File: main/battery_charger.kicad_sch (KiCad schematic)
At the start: 52 parts, among them Q401 IXTP28P065T, Q402 TK4R3E06PL, Q403 IRLML0030, Q404 FDS6681Z, Q405 FDS6681Z, Q406 IRLML0030, U401 LT8710, U402 TMCS1101, U403 TSV911xxLx

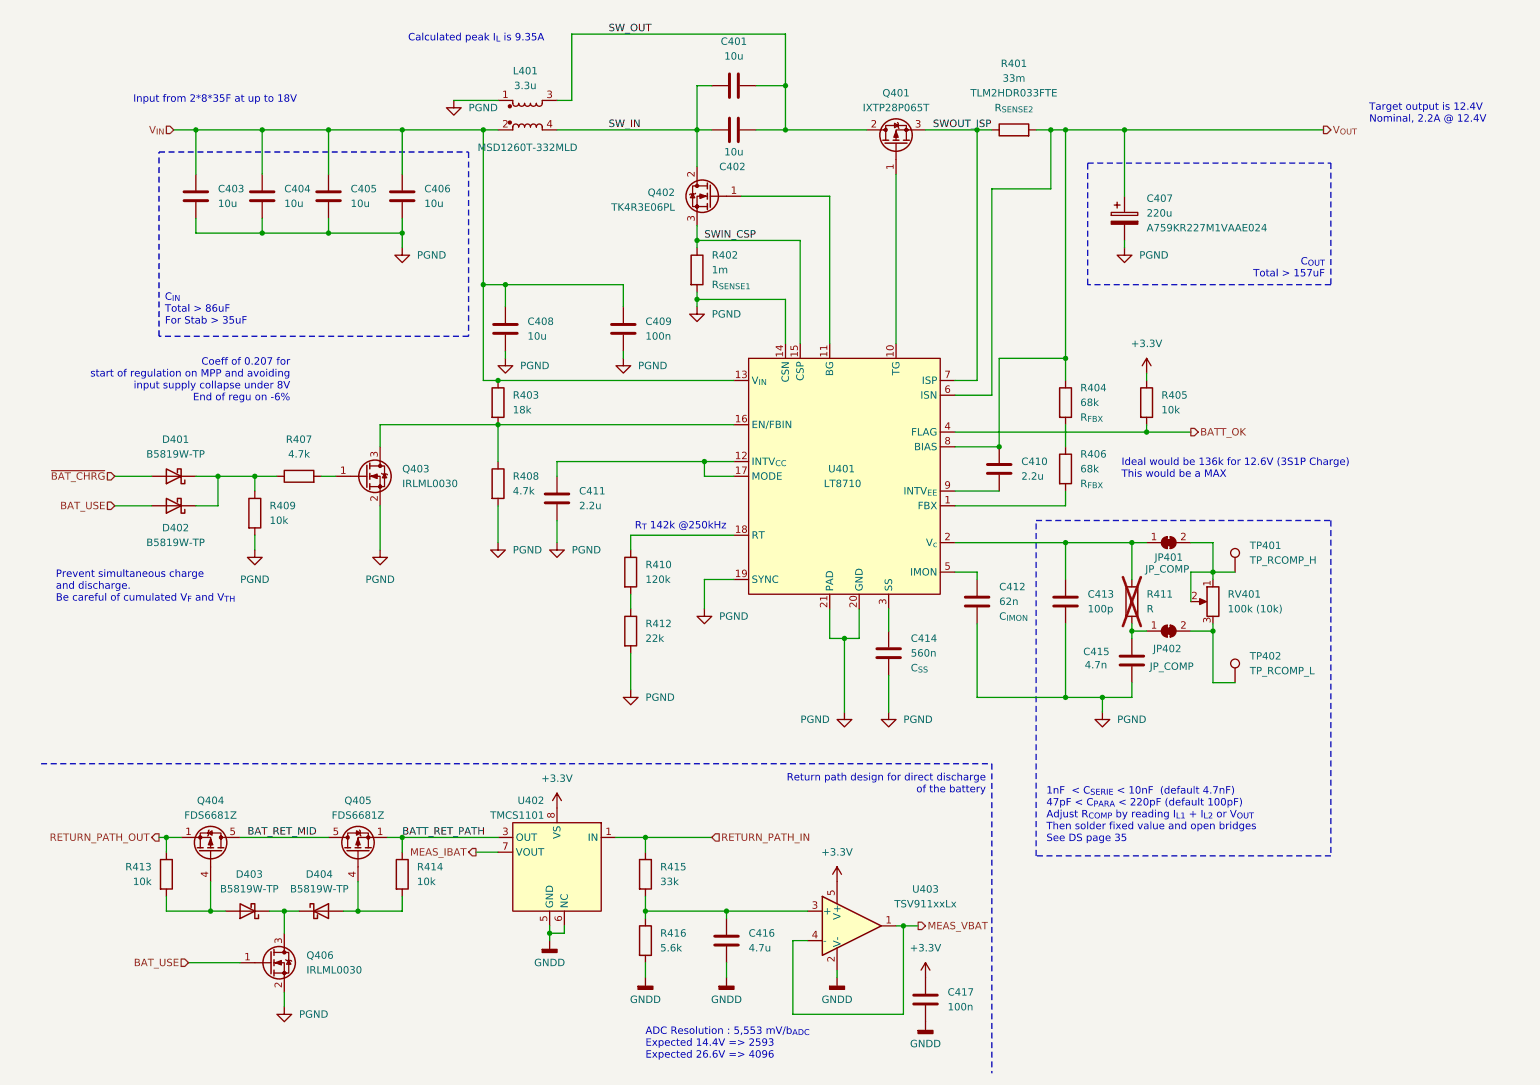
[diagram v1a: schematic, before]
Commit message: Sent to fab
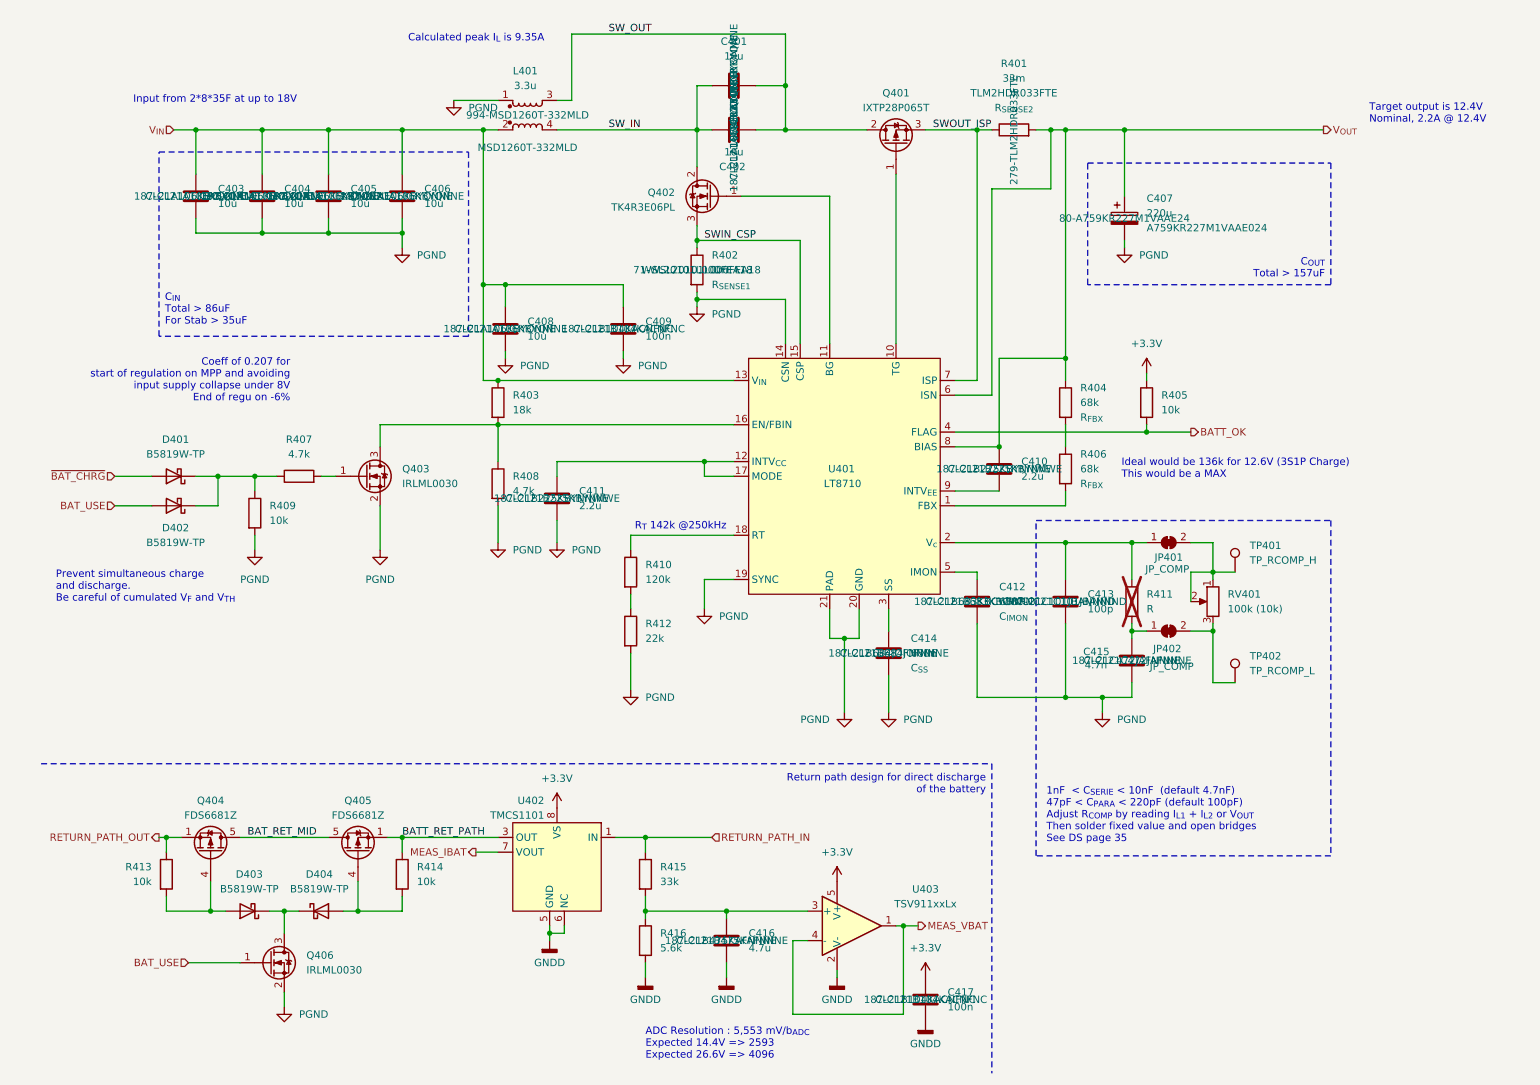
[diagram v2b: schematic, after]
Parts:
- C401, C402, C403, C404, C405, C406, C408: MPN (none) -> CL21A106KBYQNNE; Mouser SKU (none) -> 187-CL21A106KBYQNNE
- C407: Mouser SKU (none) -> 80-A759KR227M1VAAE24
- C409, C417: MPN (none) -> CL21B104KACNFNC; Mouser SKU (none) -> 187-CL21B104KACNFNC
- C410, C411: MPN (none) -> CL21B225KBYNNWE; Mouser SKU (none) -> 187-CL21B225KBYNNWE
- C412: value 62n -> 68n; MPN (none) -> CL21B683KBCWPNC; Mouser SKU (none) -> 187-CL21B683KBCWPNC
- C413: MPN (none) -> CL21C101JBANNND; Mouser SKU (none) -> 187-CL21C101JBANNND
- C414: value 560n -> 680n; MPN (none) -> CL21B684JOFNNNE; Mouser SKU (none) -> 187-CL21B684JOFNNNE
- C415: MPN (none) -> CL21C472JAFNNNE; Mouser SKU (none) -> 187-CL21C472JAFNNNE
- C416: MPN (none) -> CL21B475KAFNNNE; Mouser SKU (none) -> 187-CL21B475KAFNNNE
- L401: Mouser SKU (none) -> 994-MSD1260T-332MLD
- R401: Mouser SKU (none) -> 279-TLM2HDR033FTE
- R402: MPN (none) -> WSL20101L000FEA18; Mouser SKU (none) -> 71-WSL20101L000FEA18
